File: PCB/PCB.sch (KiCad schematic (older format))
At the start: 202 parts, among them J1 USB_mini_micro_B, K0,0 KEYSW, K0,1 KEYSW, K0,10 KEYSW, K0,11 KEYSW, K0,12 KEYSW, K0,13 KEYSW, K0,14 KEYSW, K0,15 KEYSW, K0,16 KEYSW, K0,17 KEYSW, K0,18 KEYSW, K0,19 KEYSW, K0,2 KEYSW, K0,20 KEYSW, K0,3 KEYSW, K0,4 KEYSW, K0,5 KEYSW, K0,6 KEYSW, K0,7 KEYSW, K0,8 KEYSW, K0,9 KEYSW, K1,0 KEYSW, K1,1 KEYSW, K1,10 KEYSW, K1,11 KEYSW, K1,12 KEYSW, K1,13 KEYSW, K1,14 KEYSW, K1,15 KEYSW, K1,16 KEYSW, K1,17 KEYSW, K1,18 KEYSW, K1,19 KEYSW, K1,2 KEYSW, K1,20 KEYSW, K1,3 KEYSW, K1,4 KEYSW, K1,5 KEYSW, K1,6 KEYSW, K1,7 KEYSW, K1,8 KEYSW, K1,9 KEYSW, K2,0 KEYSW, K2,1 KEYSW, K2,10 KEYSW, K2,11 KEYSW, K2,12 KEYSW, K2,13 KEYSW, K2,14 KEYSW, K2,15 KEYSW, K2,17 KEYSW, K2,18 KEYSW, K2,19 KEYSW, K2,2 KEYSW, K2,20 KEYSW, K2,4 KEYSW, K2,5 KEYSW, K2,6 KEYSW, K2,7 KEYSW, K2,8 KEYSW, K2,9 KEYSW, K3,0 KEYSW, K3,1 KEYSW, K3,10 KEYSW, K3,11 KEYSW, K3,12 KEYSW, K3,13 KEYSW, K3,14 KEYSW, K3,16 KEYSW, K3,18 KEYSW, K3,19 KEYSW, K3,2 KEYSW, K3,20 KEYSW, K3,3 KEYSW, K3,4 KEYSW, K3,5 KEYSW, K3,6 KEYSW, K3,7 KEYSW, K3,8 KEYSW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

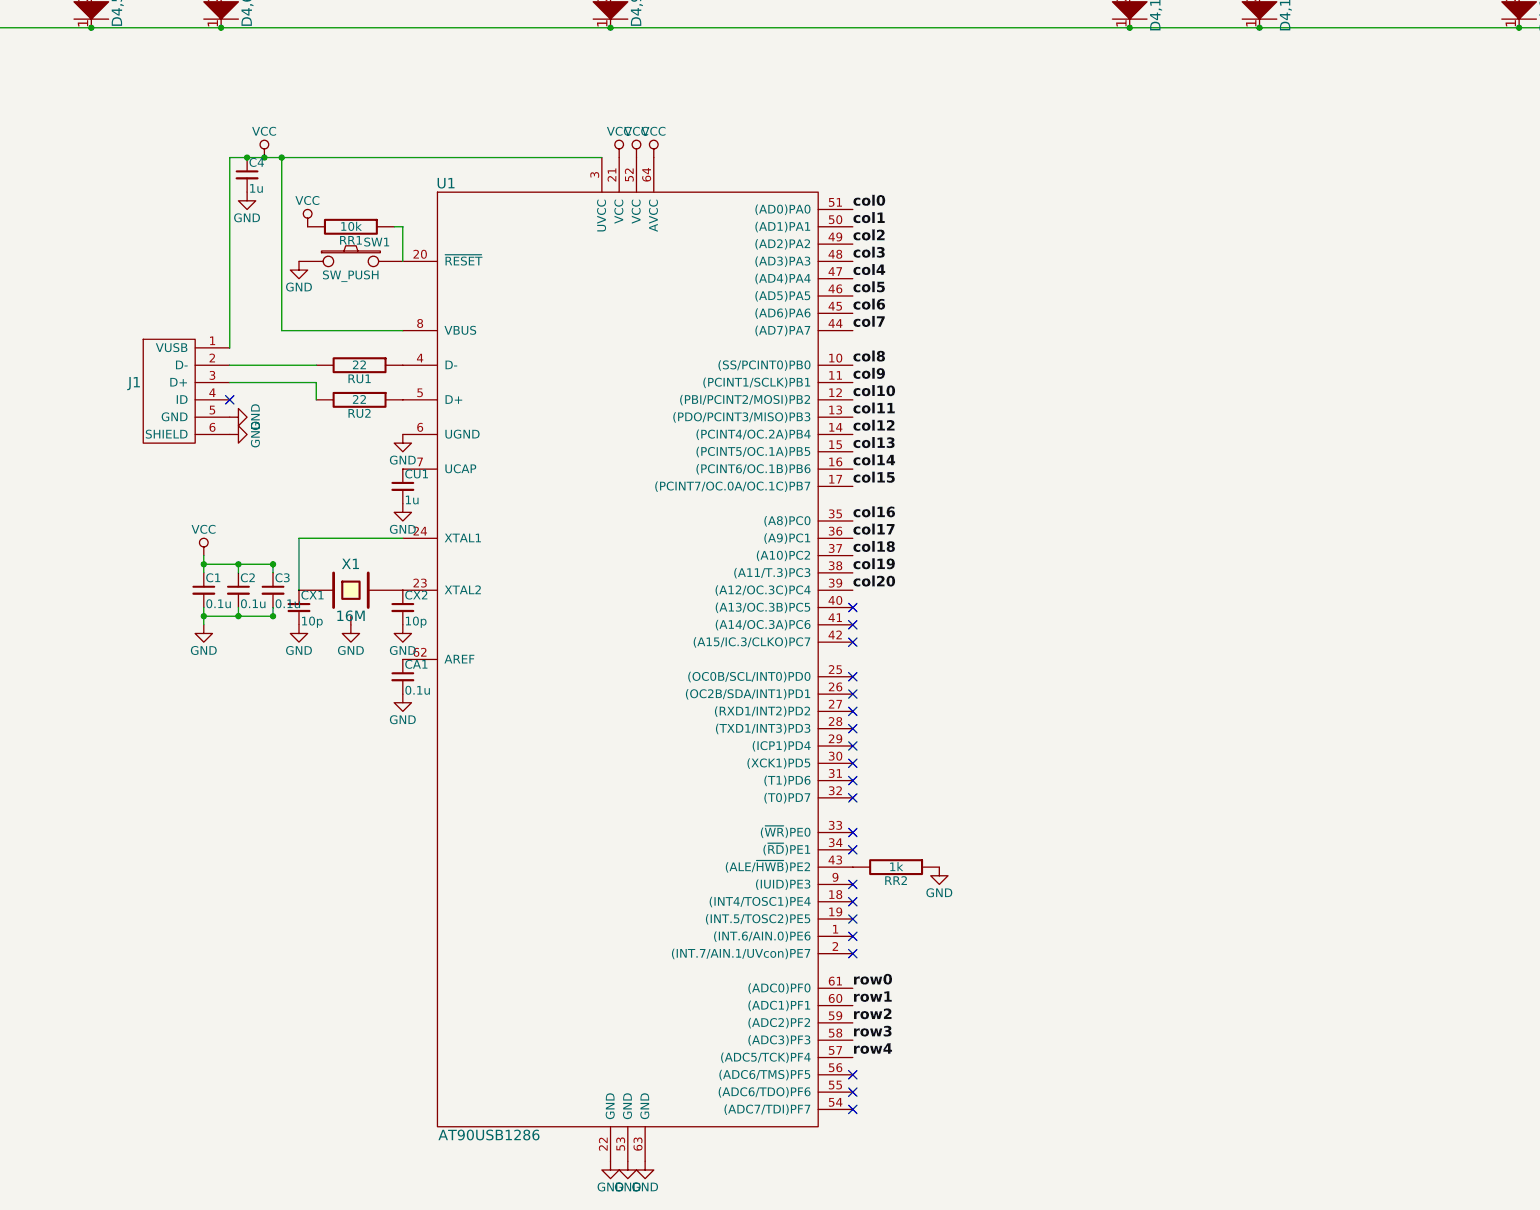
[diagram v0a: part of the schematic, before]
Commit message: Taking new design approach; updated submodules
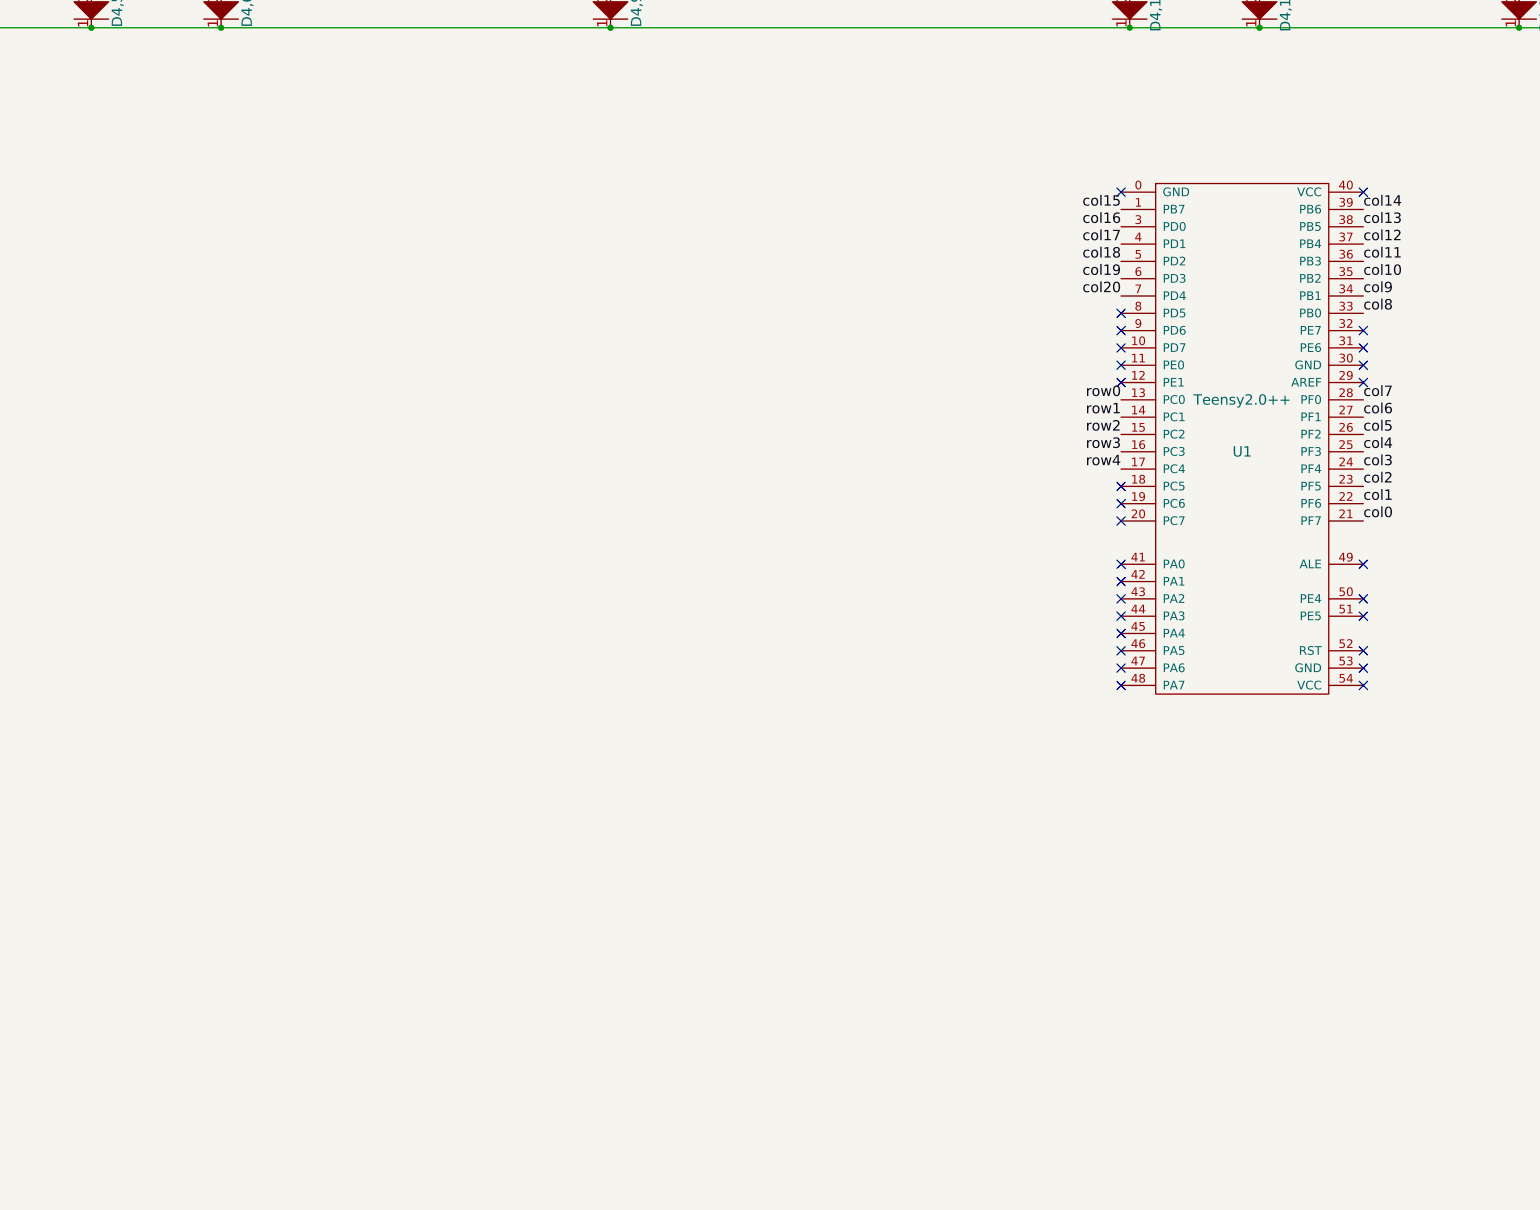
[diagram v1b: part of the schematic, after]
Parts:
- removed C1, C2, C3, CA1: 0.1u, Capacitors_SMD:C_0805_HandSoldering, symbol C_Small
- removed C4, CU1: 1u, Capacitors_SMD:C_0805_HandSoldering, symbol C_Small
- removed CX1, CX2: 10p, Capacitors_SMD:C_0805_HandSoldering, symbol C_Small
- removed J1: USB_mini_micro_B, keyboard_parts:USB_miniB_hirose_5S8, symbol USB_mini_micro_B
- removed RR1: 10k, Resistors_SMD:R_0805_HandSoldering, symbol R
- removed RR2: 1k, Resistors_SMD:R_0805_HandSoldering, symbol R
- removed RU1, RU2: 22, Resistors_SMD:R_0805_HandSoldering, symbol R
- removed SW1: SW_PUSH, Buttons_Switches_SMD:SW_SPST_TL3342, symbol SW_PUSH
- removed U1: AT90USB1286, Housings_QFP:TQFP-64_14x14mm_Pitch0.8mm, symbol AT90USB1286
- removed X1: 16M, keyboard_parts:FA-238, symbol XTAL_GND
- added U1: Teensy2.0++, keebs:Teensy_20, symbol Teensy2.0++
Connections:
- net col0: now also U1.21 (PF7)
- net col1: now also U1.22 (PF6)
- net col10: now also U1.35 (PB2)
- net col11: now also U1.36 (PB3)
- net col12: now also U1.37 (PB4)
- net col13: now also U1.38 (PB5)
- net col14: now also U1.39 (PB6)
- net col15: now also U1.1 (PB7)
- net col16: now also U1.3 (PD0)
- net col17: now also U1.4 (PD1)
- net col18: now also U1.5 (PD2)
- net col19: now also U1.6 (PD3)
- net col2: now also U1.23 (PF5)
- net col20: now also U1.7 (PD4)
- net col3: now also U1.24 (PF4)
- net col4: now also U1.25 (PF3)
- net col5: now also U1.26 (PF2)
- net col6: now also U1.27 (PF1)
- net col7: now also U1.28 (PF0)
- net col8: now also U1.33 (PB0)
- net col9: now also U1.34 (PB1)
- net row0: now also U1.13 (PC0)
- net row1: now also U1.14 (PC1)
- net row2: now also U1.15 (PC2)
- net row3: now also U1.16 (PC3)
- net row4: now also U1.17 (PC4)
- no-connect marks 22 -> 28

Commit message: 2017.11.08 Update
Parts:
- removed U1: Teensy2.0++, keebs:Teensy_20, symbol Teensy2.0++
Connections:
- no-connect marks 28 -> 0
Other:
- moved on the sheet: D0,0, D0,1, D0,10, D0,11, D0,12, D0,13, D0,14, D0,15, D0,16, D0,17, D0,18, D0,19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
